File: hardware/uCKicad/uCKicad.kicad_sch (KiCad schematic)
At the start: 23 parts, among them J1 Conn_02x07_Odd_Even, J2 INPUT, J3 OUTPUT, J4 POWER, U1 MCP1802x-xx02xOT, U2 MCP4801, U3 STM32L021K4Tx

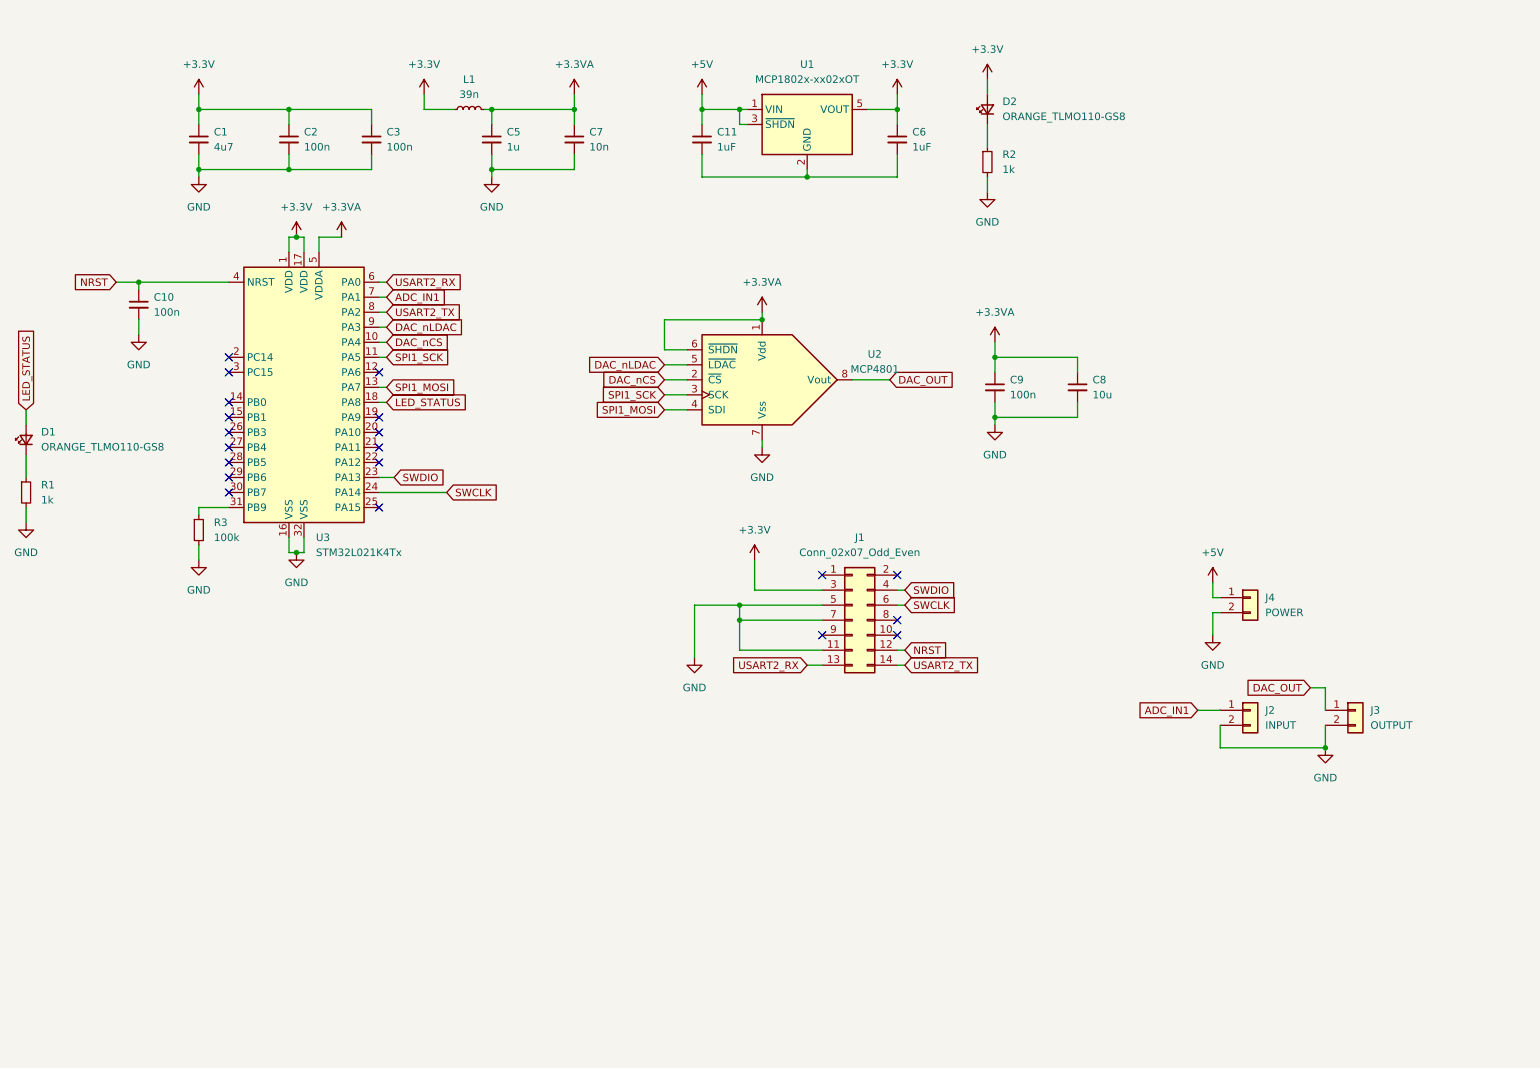
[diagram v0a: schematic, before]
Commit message: on essaie de sauver le PC
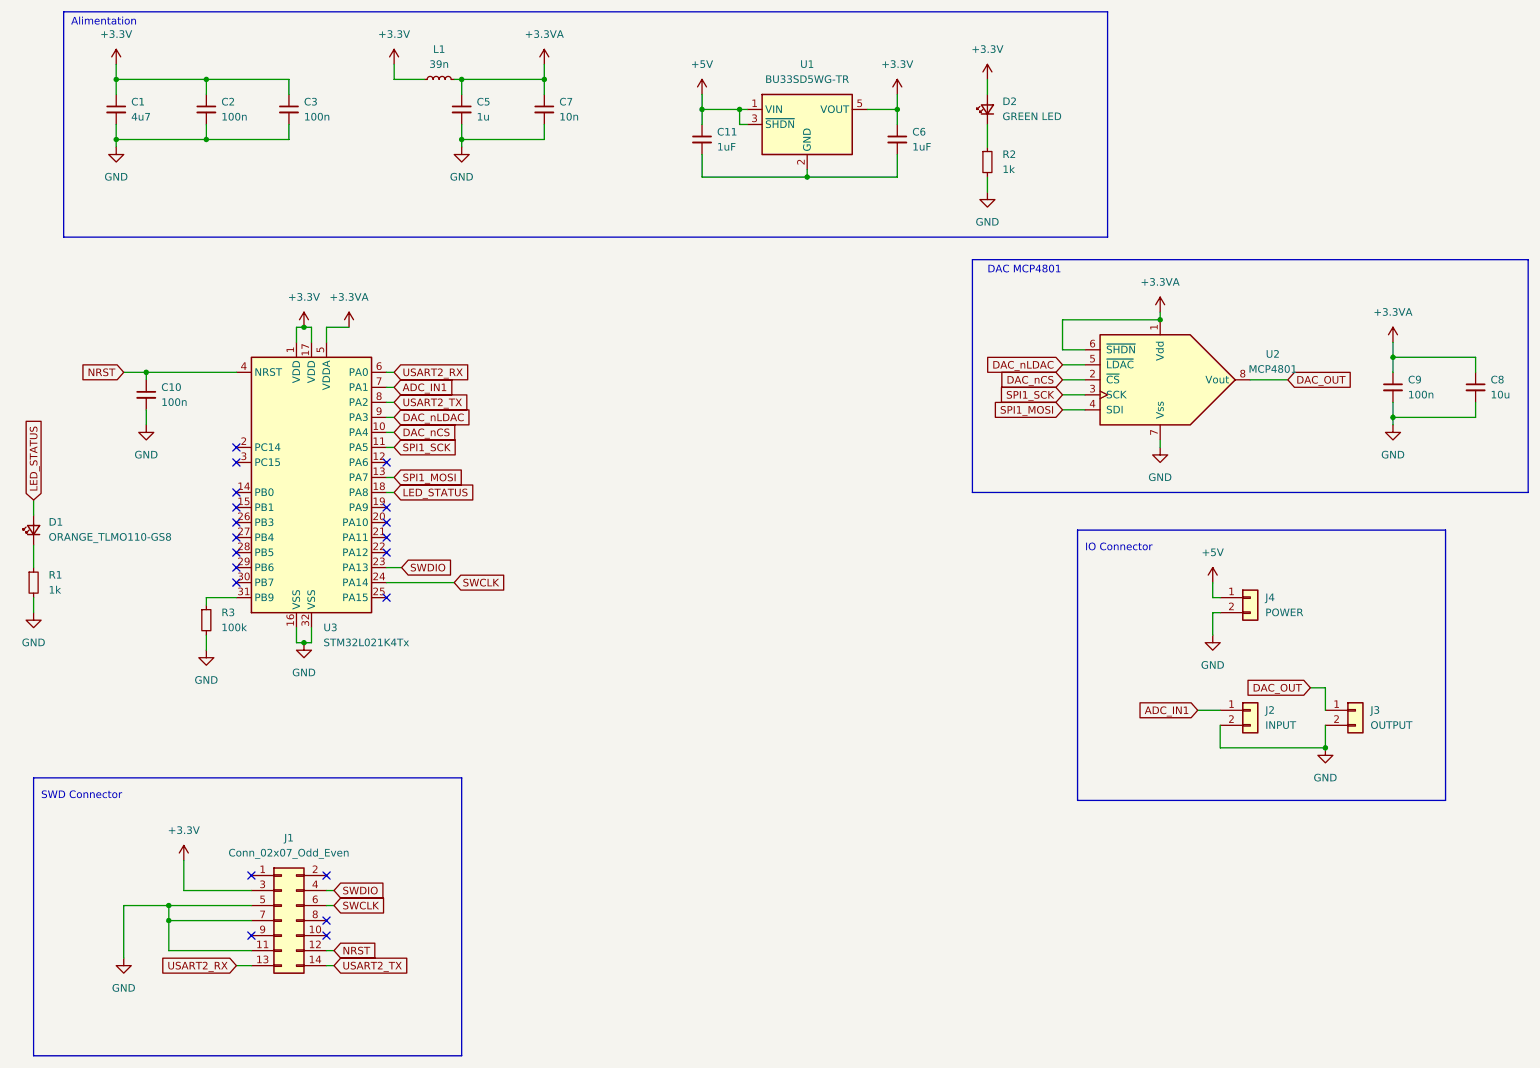
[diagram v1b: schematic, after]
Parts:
- C1, C10, C2, C3, C5, C7, C9: footprint (none) -> Capacitor_SMD:C_0805_2012Metric_Pad1.18x1.45mm_HandSolder
- C11, C6, C8: footprint (none) -> Capacitor_SMD:C_0805_2012Metric
- D1: footprint (none) -> LED_SMD:LED_0603_1608Metric_Pad1.05x0.95mm_HandSolder
- D2: value ORANGE_TLMO110-GS8 -> GREEN LED; footprint (none) -> LED_SMD:LED_0603_1608Metric_Pad1.05x0.95mm_HandSolder
- J1: footprint (none) -> Connector_PinHeader_1.27mm:PinHeader_2x07_P1.27mm_Vertical_SMD
- J2, J3, J4: footprint (none) -> Connector_JST:JST_XH_B2B-XH-A_1x02_P2.50mm_Vertical
- L1: footprint (none) -> Inductor_SMD:L_0805_2012Metric_Pad1.05x1.20mm_HandSolder
- R1, R2, R3: footprint (none) -> Resistor_SMD:R_0805_2012Metric_Pad1.20x1.40mm_HandSolder
- U1: value MCP1802x-xx02xOT -> BU33SD5WG-TR
- U2: footprint (none) -> Package_SO:SOIC-8_3.9x4.9mm_P1.27mm
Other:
- note added: "Alimentation"
- note added: "DAC MCP4801"
- note added: "IO Connector"
- note added: "SWD Connector"
- moved on the sheet: C1, C10, C2, C3, C5, C7, C8, C9, D1, J1, L1, R1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
